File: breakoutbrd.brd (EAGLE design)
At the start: 71.1 x 96.5 mm, 7 parts

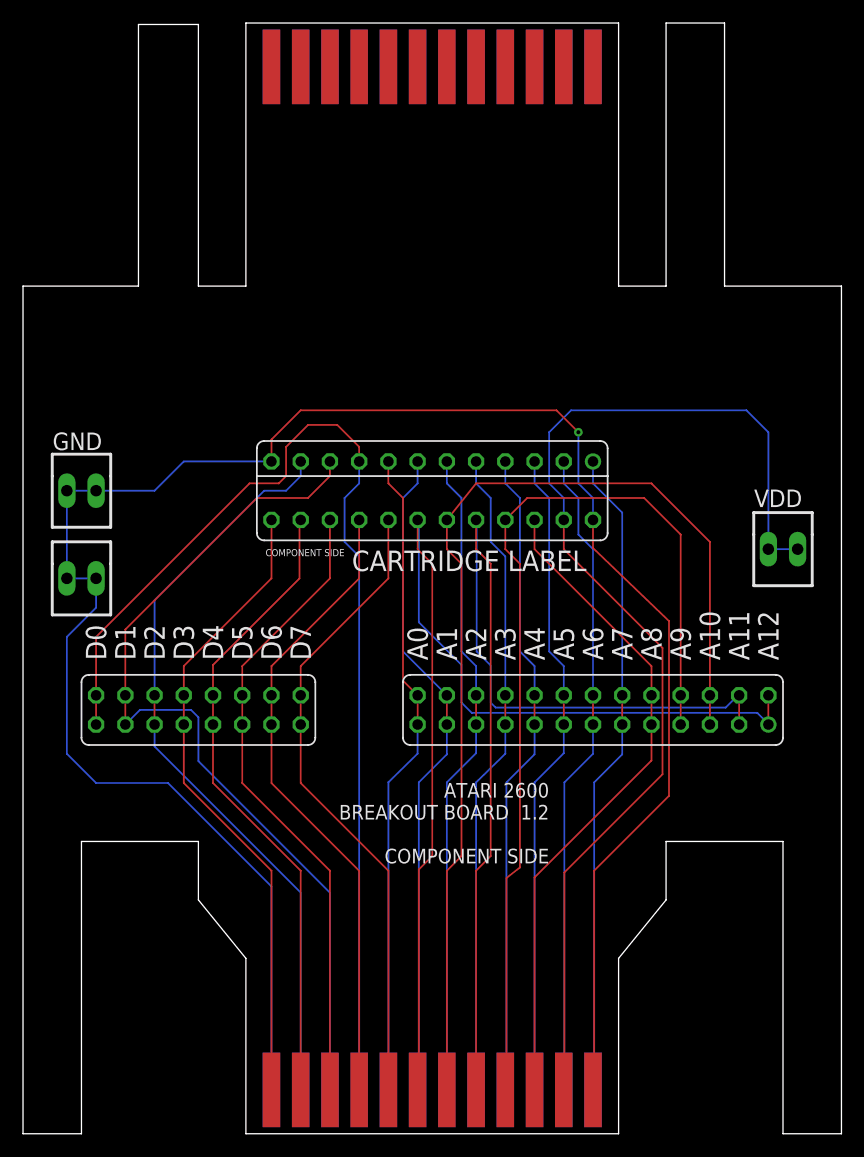
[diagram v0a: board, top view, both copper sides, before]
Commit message: more layout work
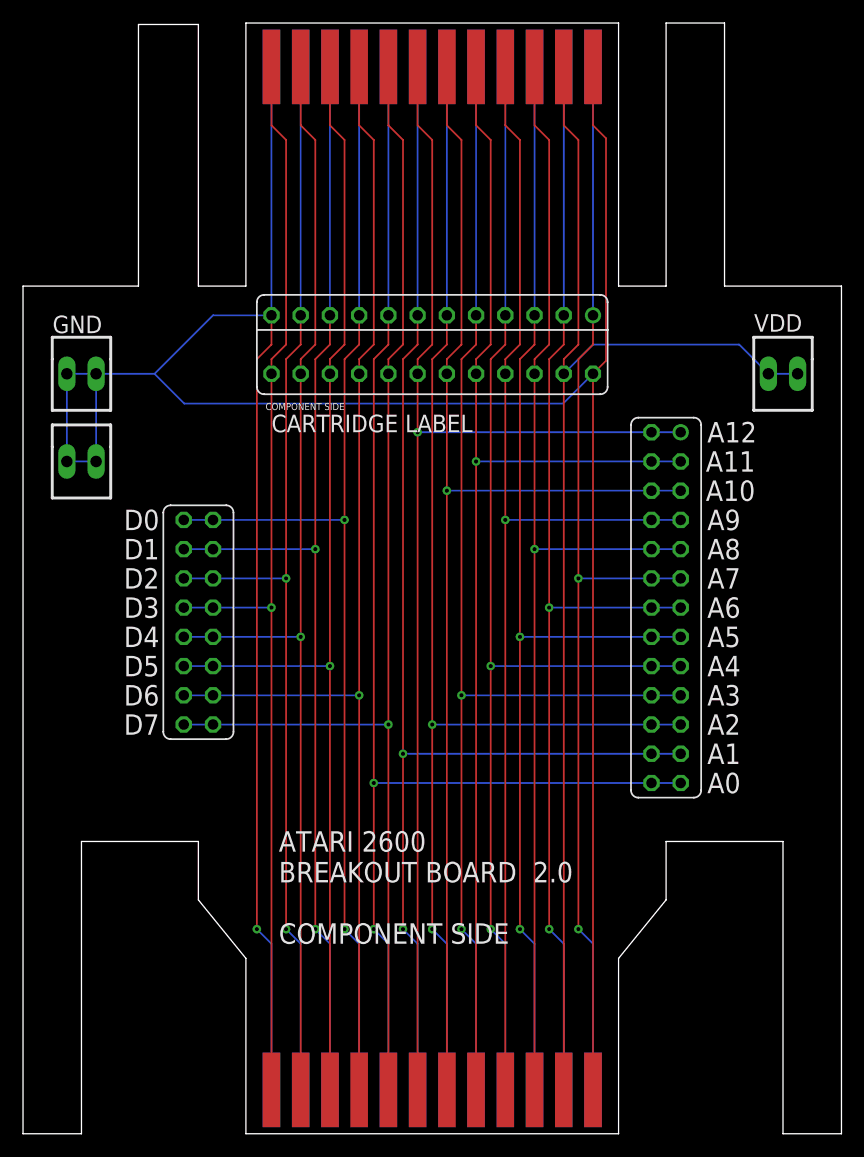
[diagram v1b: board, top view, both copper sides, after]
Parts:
- moved VDD 15.2 mm to (67.3, 66.0)
- moved U$1 12.7 mm to (36.8, 68.6)
- moved SV2 10.9 mm to (57.1, 45.7), turned to 270 degrees
- moved GND 10.2 mm to (6.35, 66.0)
- moved GND1 10.2 mm to (6.35, 58.4)
- moved SV1 7.62 mm to (16.5, 44.5), turned to 90 degrees
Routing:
- net GND: track 179.2 -> 257.7 mm
- net CADDR0: track 56.7 -> 116.6 mm, vias 0 -> 2
- net CADDR1: track 57.8 -> 114.1 mm, vias 0 -> 2
- net CADDR2: track 56.7 -> 111.5 mm, vias 0 -> 2
- net CADDR3: track 56.7 -> 109.0 mm, vias 0 -> 2
- net CDATA7: track 55.8 -> 107.7 mm, vias 0 -> 1
- net CADDR4: track 56.8 -> 106.5 mm, vias 0 -> 2
- net CDATA6: track 55.8 -> 105.2 mm, vias 0 -> 1
- net CADDR5: track 56.7 -> 103.9 mm, vias 0 -> 2
- net CDATA5: track 55.8 -> 102.7 mm, vias 0 -> 1
- net CADDR8: track 57.9 -> 102.7 mm, vias 0 -> 1
- net CADDR6: track 56.7 -> 101.4 mm, vias 0 -> 2
- net CDATA4: track 55.9 -> 100.1 mm, vias 0 -> 1
- net CADDR7: track 56.8 -> 98.8 mm, vias 0 -> 2
- net CDATA3: track 55.8 -> 97.6 mm, vias 0 -> 1
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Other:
- board text added: "ATARI 2600 BREAKOUT BOARD 2.0 COMPONENT SIDE"
- board text removed: "ATARI 2600 BREAKOUT BOARD 1.2 COMPONENT SIDE"
